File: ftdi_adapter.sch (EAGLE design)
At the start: 4 parts, among them J2 UPDI COMPACT, J3 6PIN SERIAL

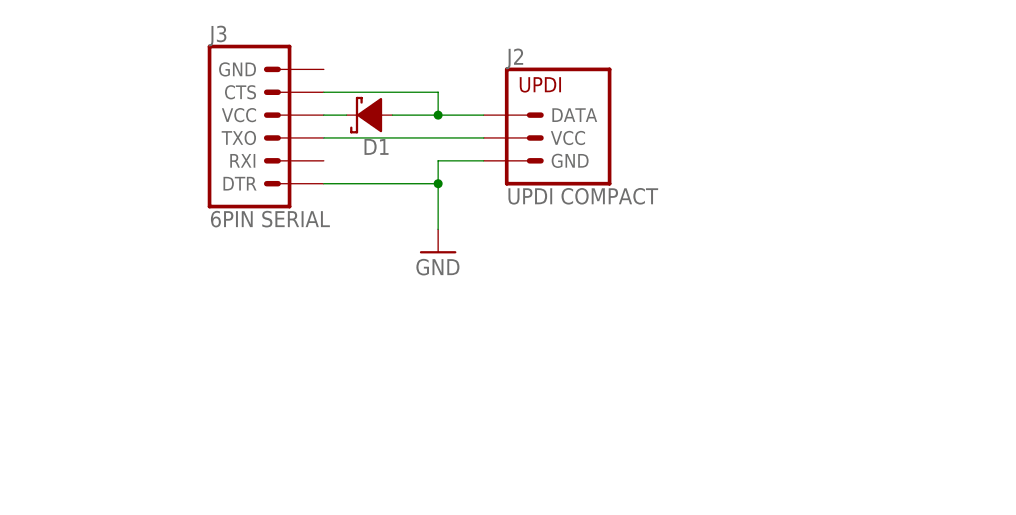
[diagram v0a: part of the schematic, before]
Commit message: initial version
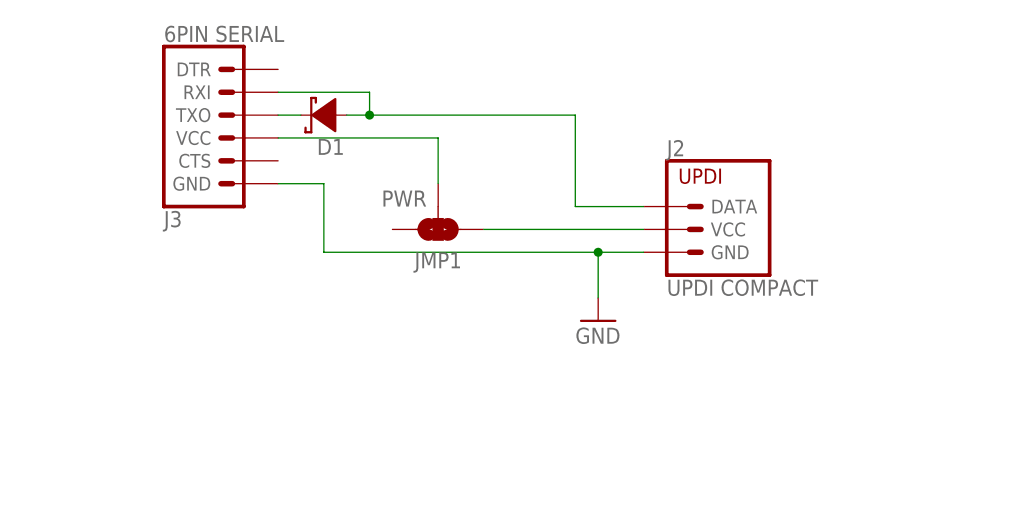
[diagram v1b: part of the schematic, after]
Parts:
- added JMP1: PWR, bt:JUMPER-2-WAY-PTH-0.1IN
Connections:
- new net DATA: D1.A, J2.DATA, J3.RXI
- net GND: now also J3.GND; no longer J3.DTR
- net N$1: now also J3.TXO; no longer J3.VCC
- net N$2: now also J3.VCC, JMP1.2; no longer D1.A, J2.DATA, J3.CTS
- net VCC: now also JMP1.1; no longer J3.TXO
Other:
- moved on the sheet: D1, J2, J3
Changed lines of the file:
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@@
 <part name="U$1" library="bt" deviceset="BTLOGO" device="-LOGO-SM"/>
 <part name="J3" library="bt_communication" deviceset="6PIN_TARGET" device="_LEFT" value="6PIN SERIAL"/>
+<part name="JMP1" library="bt" deviceset="JUMPER-2-WAY" device="-PTH-0.1IN" value="PWR"/>
 </parts>
 <sheets>
@@
 </plain>
 <instances>
-<instance part="J2" gate="J1" x="134.62" y="101.6"/>
-<instance part="D1" gate="A" x="114.3" y="104.14" rot="R180"/>
+<instance part="J2" gate="J1" x="152.4" y="91.44"/>
+<instance part="D1" gate="A" x="109.22" y="104.14" rot="R180"/>
 <instance part="FRAME1" gate="G$1" x="0" y="0"/>
 <instance part="FRAME1" gate="G$2" x="147.32" y="2.54"/>
-<instance part="GND1" gate="1" x="121.92" y="88.9"/>
+<instance part="GND1" gate="1" x="139.7" y="81.28"/>
 <instance part="U$1" gate="G$1" x="5.08" y="5.08"/>
-<instance part="J3" gate="J1" x="104.14" y="101.6"/>
+<instance part="J3" gate="J1" x="99.06" y="104.14" rot="MR180"/>
+<instance part="JMP1" gate="J1" x="121.92" y="91.44" rot="R180"/>
 </instances>
 <busses>
 </busses>
 <nets>
-<net name="N$2" class="0">
-<segment>
-<wire x1="109.22" y1="106.68" x2="121.92" y2="106.68" width="0.1524" layer="91"/>
-<wire x1="121.92" y1="106.68" x2="121.92" y2="104.14" width="0.1524" layer="91"/>
-<pinref part="J2" gate="J1" pin="DATA"/>
-<wire x1="121.92" y1="104.14" x2="127" y2="104.14" width="0.1524" layer="91"/>
-<pinref part="D1" gate="A" pin="A"/>
-<wire x1="116.84" y1="104.14" x2="121.92" y2="104.14" width="0.1524" layer="91"/>
-<junction x="121.92" y="104.14"/>
-<pinref part="J3" gate="J1" pin="CTS"/>
-</segment>
-</net>
 <net name="VCC" class="0">
 <segment>
 <pinref part="J2" gate="J1" pin="VCC"/>
-<wire x1="127" y1="101.6" x2="109.22" y2="101.6" width="0.1524" layer="91"/>
-<pinref part="J3" gate="J1" pin="TXO"/>
-</segment>
-</net>
-<net name="N$1" class="0">
-<segment>
-<pinref part="D1" gate="A" pin="C"/>
-<wire x1="111.76" y1="104.14" x2="109.22" y2="104.14" width="0.1524" layer="91"/>
-<pinref part="J3" gate="J1" pin="VCC"/>
+<wire x1="127" y1="91.44" x2="144.78" y2="91.44" width="0.1524" layer="91"/>
+<pinref part="JMP1" gate="J1" pin="1"/>
 </segment>
 </net>
@@
 <segment>
 <pinref part="J2" gate="J1" pin="GND"/>
-<wire x1="127" y1="99.06" x2="121.92" y2="99.06" width="0.1524" layer="91"/>
-<wire x1="121.92" y1="99.06" x2="121.92" y2="96.52" width="0.1524" layer="91"/>
-<wire x1="121.92" y1="96.52" x2="109.22" y2="96.52" width="0.1524" layer="91"/>
+<wire x1="144.78" y1="88.9" x2="139.7" y2="88.9" width="0.1524" layer="91"/>
 <pinref part="GND1" gate="1" pin="GND"/>
-<wire x1="121.92" y1="91.44" x2="121.92" y2="96.52" width="0.1524" layer="91"/>
-<junction x="121.92" y="96.52"/>
-<pinref part="J3" gate="J1" pin="DTR"/>
+<wire x1="139.7" y1="83.82" x2="139.7" y2="88.9" width="0.1524" layer="91"/>
+<junction x="139.7" y="88.9"/>
+<pinref part="J3" gate="J1" pin="GND"/>
+<wire x1="104.14" y1="96.52" x2="109.22" y2="96.52" width="0.1524" layer="91"/>
+<wire x1="109.22" y1="96.52" x2="109.22" y2="88.9" width="0.1524" layer="91"/>
+<wire x1="109.22" y1="88.9" x2="139.7" y2="88.9" width="0.1524" layer="91"/>
 </segment>
 </net>
+<net name="N$1" class="0">
+<segment>
+<pinref part="J3" gate="J1" pin="TXO"/>
+<pinref part="D1" gate="A" pin="C"/>
+<wire x1="106.68" y1="104.14" x2="104.14" y2="104.14" width="0.1524" layer="91"/>
+</segment>
+</net>
+<net name="DATA" class="0">
+<segment>
+<pinref part="J3" gate="J1" pin="RXI"/>
+<wire x1="104.14" y1="106.68" x2="114.3" y2="106.68" width="0.1524" layer="91"/>
+<wire x1="114.3" y1="106.68" x2="114.3" y2="104.14" width="0.1524" layer="91"/>
+<pinref part="D1" gate="A" pin="A"/>
+<wire x1="114.3" y1="104.14" x2="111.76" y2="104.14" width="0.1524" layer="91"/>
+<pinref part="J2" gate="J1" pin="DATA"/>
+<wire x1="144.78" y1="93.98" x2="137.16" y2="93.98" width="0.1524" layer="91"/>
+<wire x1="137.16" y1="93.98" x2="137.16" y2="104.14" width="0.1524" layer="91"/>
+<wire x1="114.3" y1="104.14" x2="137.16" y2="104.14" width="0.1524" layer="91"/>
+<junction x="114.3" y="104.14"/>
+</segment>
+</net>
+<net name="N$2" class="0">
+<segment>
+<pinref part="J3" gate="J1" pin="VCC"/>
+<pinref part="JMP1" gate="J1" pin="2"/>
+<wire x1="104.14" y1="101.6" x2="121.92" y2="101.6" width="0.1524" layer="91"/>
+<wire x1="121.92" y1="101.6" x2="121.92" y2="96.52" width="0.1524" layer="91"/>
+</segment>
+</net>
